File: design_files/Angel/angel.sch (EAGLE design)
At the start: 10 parts

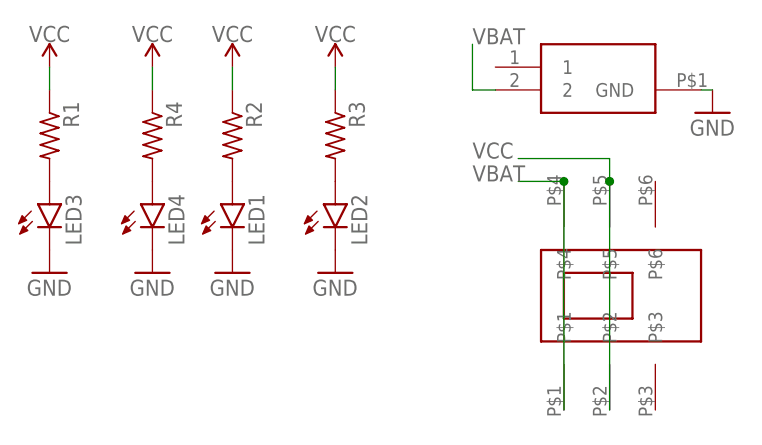
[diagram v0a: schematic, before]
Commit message: adds updates and pics
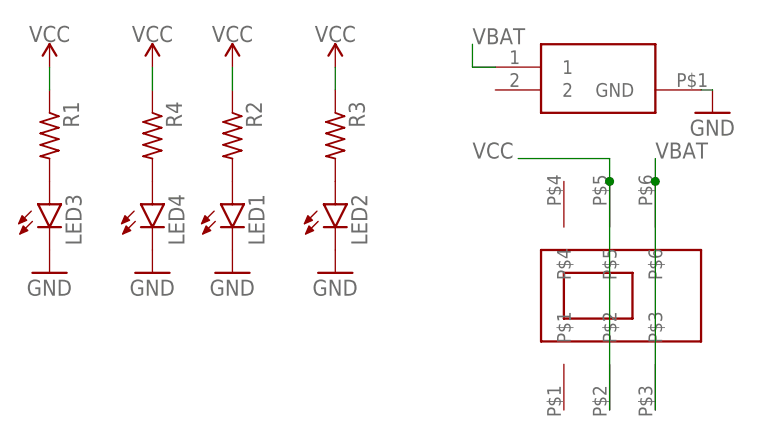
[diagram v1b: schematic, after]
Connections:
- net VBAT: now also U$1.P$3, U$1.P$6, VBAT.1; no longer U$1.P$1, U$1.P$4, VBAT.2
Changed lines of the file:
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@@
 <part name="SUPPLY1" library="SparkFun-PowerSymbols" deviceset="VCC" device=""/>
 <part name="SUPPLY2" library="SparkFun-PowerSymbols" deviceset="VCC" device=""/>
-<part name="VBAT" library="SamacSys_Parts" deviceset="BAT-HLD-012-SMT" device="" override_package3d_urn="urn:adsk.eagle:package:15679619/3" override_package_urn="urn:adsk.eagle:footprint:15679620/1" override_locally_modified="yes"/>
+<part name="VBAT" library="SamacSys_Parts" deviceset="BAT-HLD-012-SMT" device="" override_package3d_urn="urn:adsk.eagle:package:32575048/5" override_package_urn="urn:adsk.eagle:footprint:32575049/1"/>
 <part name="GND3" library="supply1" library_urn="urn:adsk.eagle:library:371" deviceset="GND" device=""/>
-<part name="U$1" library="electroninks" deviceset="CL-SB-22A-02T-SLIDE-SWITCH-TUCKED-PADS" device="" override_package3d_urn="urn:adsk.eagle:package:15679591/3" override_package_urn="urn:adsk.eagle:footprint:15679592/1"/>
+<part name="U$1" library="electroninks" deviceset="CL-SB-22A-02T-SLIDE-SWITCH-TUCKED-PADS" device="" override_package3d_urn="urn:adsk.eagle:package:32575056/3" override_package_urn="urn:adsk.eagle:footprint:32575057/1"/>
 <part name="LED3" library="led" library_urn="urn:adsk.eagle:library:259" deviceset="LED" device="CHIP-LED0805" package3d_urn="urn:adsk.eagle:package:15818/2"/>
 <part name="LED4" library="led" library_urn="urn:adsk.eagle:library:259" deviceset="LED" device="CHIP-LED0805" package3d_urn="urn:adsk.eagle:package:15818/2"/>
@@
 <label x="71.12" y="-5.08" size="1.778" layer="95"/>
 <pinref part="U$1" gate="G$1" pin="P$2"/>
-<wire x1="86.36" y1="-7.62" x2="86.36" y2="-33.02" width="0.1524" layer="91"/>
+<wire x1="86.36" y1="-33.02" x2="86.36" y2="-7.62" width="0.1524" layer="91"/>
 <junction x="86.36" y="-7.62"/>
 </segment>
@@
 <net name="VBAT" class="0">
 <segment>
-<pinref part="U$1" gate="G$1" pin="P$4"/>
-<wire x1="81.28" y1="-7.62" x2="76.2" y2="-7.62" width="0.1524" layer="91"/>
-<label x="71.12" y="-7.62" size="1.778" layer="95"/>
-<pinref part="U$1" gate="G$1" pin="P$1"/>
-<wire x1="81.28" y1="-33.02" x2="81.28" y2="-7.62" width="0.1524" layer="91"/>
-<junction x="81.28" y="-7.62"/>
+<label x="71.12" y="7.62" size="1.778" layer="95"/>
+<pinref part="VBAT" gate="G$1" pin="1"/>
+<wire x1="71.12" y1="5.08" x2="71.12" y2="7.62" width="0.1524" layer="91"/>
+<wire x1="73.66" y1="5.08" x2="71.12" y2="5.08" width="0.1524" layer="91"/>
 </segment>
 <segment>
-<pinref part="VBAT" gate="G$1" pin="2"/>
-<wire x1="73.66" y1="2.54" x2="71.12" y2="2.54" width="0.1524" layer="91"/>
-<wire x1="71.12" y1="2.54" x2="71.12" y2="7.62" width="0.1524" layer="91"/>
-<label x="71.12" y="7.62" size="1.778" layer="95"/>
+<wire x1="91.44" y1="-7.62" x2="91.44" y2="-5.08" width="0.1524" layer="91"/>
+<pinref part="U$1" gate="G$1" pin="P$6"/>
+<label x="91.44" y="-5.08" size="1.778" layer="95"/>
+<pinref part="U$1" gate="G$1" pin="P$3"/>
+<wire x1="91.44" y1="-33.02" x2="91.44" y2="-7.62" width="0.1524" layer="91"/>
+<junction x="91.44" y="-7.62"/>
 </segment>
 </net>
